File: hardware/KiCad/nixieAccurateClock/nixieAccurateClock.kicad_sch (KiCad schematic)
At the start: 19 parts, among them J1 Conn_01x02_Pin, J2 Conn_01x02_Pin, J3 Conn_01x02_Pin, J4 Conn_01x02_Pin, SW1 SW_DIP_x08, U1 MCP23008-xSO, U2 pico iCE, U3 LTR-329ALS-01

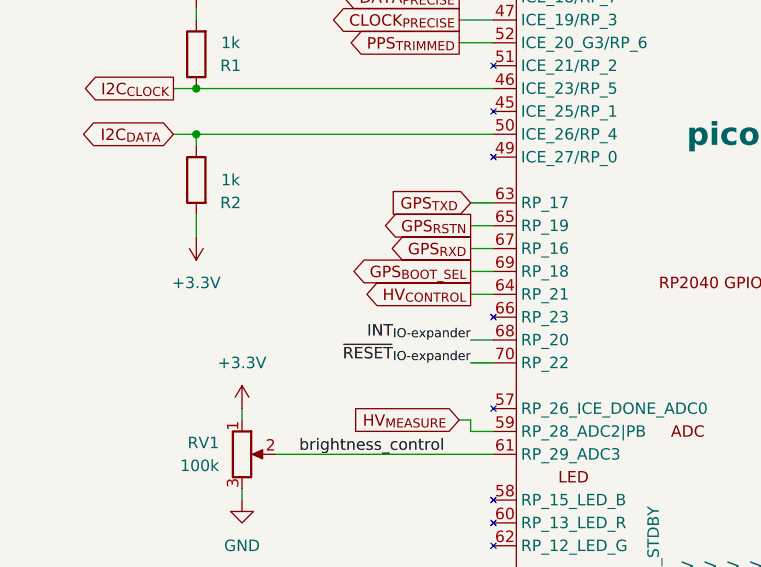
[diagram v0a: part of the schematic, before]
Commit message: WIP pinout config
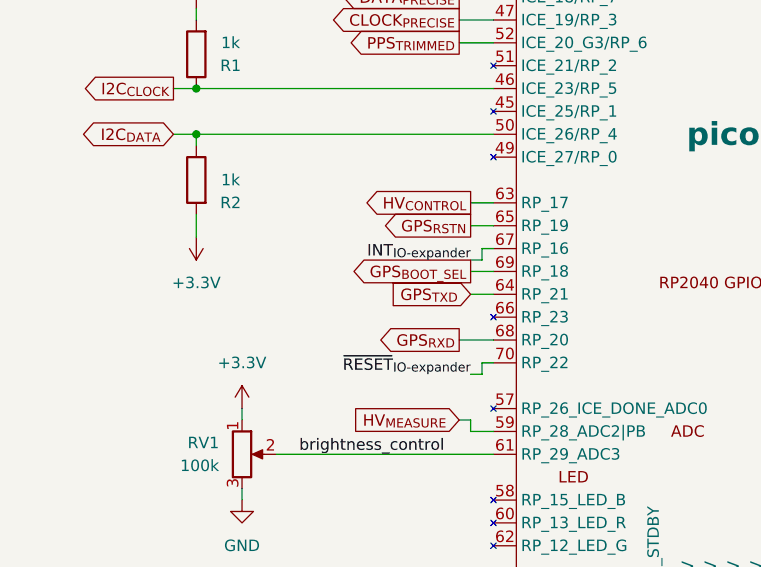
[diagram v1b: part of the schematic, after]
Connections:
- net GPS_{RXD}: now also U2.68 (RP_20); no longer U2.67 (RP_16)
- net GPS_{TXD}: now also U2.64 (RP_21); no longer U2.63 (RP_17)
- net HV_{CONTROL}: now also U2.63 (RP_17); no longer U2.64 (RP_21)
- net INT_{IO-expander}: now also U2.67 (RP_16); no longer U2.68 (RP_20)
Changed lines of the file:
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@@
   (junction (at 114.3 21.59) (diameter 0) (color 0 0 0 0)
   )
+  (wire (pts (xy 73.66 74.93) (xy 73.66 73.66))
+    (stroke (width 0) (type default))
+  )
   (wire (pts (xy 116.84 21.59) (xy 119.38 21.59))
     (stroke (width 0) (type default))
@@
     (stroke (width 0) (type default))
   )
+  (wire (pts (xy 73.66 87.63) (xy 73.66 86.36))
+    (stroke (width 0) (type default))
+  )
   (wire (pts (xy 264.16 34.29) (xy 264.16 36.83))
     (stroke (width 0) (type default))
   )
-  (wire (pts (xy 72.39 83.82) (xy 74.93 83.82))
-    (stroke (width 0) (type default))
-  )
   (wire (pts (xy 207.01 62.23) (xy 207.01 64.77))
     (stroke (width 0) (type default))
@@
     (stroke (width 0) (type default))
   )
+  (wire (pts (xy 72.39 74.93) (xy 73.66 74.93))
+    (stroke (width 0) (type default))
+  )
   (wire (pts (xy 149.86 96.52) (xy 137.16 96.52))
     (stroke (width 0) (type default))
@@
     (stroke (width 0) (type default))
   )
+  (wire (pts (xy 73.66 73.66) (xy 74.93 73.66))
+    (stroke (width 0) (type default))
+  )
   (wire (pts (xy 191.77 49.53) (xy 194.31 49.53))
     (stroke (width 0) (type default))
@@
     (stroke (width 0) (type default))
   )
+  (wire (pts (xy 72.39 78.74) (xy 74.93 78.74))
+    (stroke (width 0) (type default))
+  )
   (wire (pts (xy 92.71 137.16) (xy 92.71 140.97))
     (stroke (width 0) (type default))
@@
     (stroke (width 0) (type default))
   )
-  (wire (pts (xy 72.39 73.66) (xy 74.93 73.66))
-    (stroke (width 0) (type default))
-  )
   (wire (pts (xy 114.3 21.59) (xy 116.84 21.59))
     (stroke (width 0) (type default))
@@
     (stroke (width 0) (type default))
   )
-  (wire (pts (xy 72.39 86.36) (xy 74.93 86.36))
+  (wire (pts (xy 72.39 87.63) (xy 73.66 87.63))
     (stroke (width 0) (type default))
   )
@@
     (stroke (width 0) (type default))
   )
+  (wire (pts (xy 73.66 86.36) (xy 74.93 86.36))
+    (stroke (width 0) (type default))
+  )
+  (wire (pts (xy 71.12 83.82) (xy 74.93 83.82))
+    (stroke (width 0) (type default))
+  )
   (wire (pts (xy 71.12 45.72) (xy 74.93 45.72))
     (stroke (width 0) (type default))
@@
     (stroke (width 0) (type default))
   )
-  (wire (pts (xy 72.39 78.74) (xy 74.93 78.74))
-    (stroke (width 0) (type default))
-  )
   (wire (pts (xy 99.06 21.59) (xy 99.06 22.86))
     (stroke (width 0) (type default))
@@
     (stroke (width 0) (type default))
   )
+  (wire (pts (xy 46.99 91.44) (xy 46.99 92.71))
+    (stroke (width 0) (type default))
+  )
+  (wire (pts (xy 109.22 21.59) (xy 109.22 22.86))
+    (stroke (width 0) (type default))
+  )
+  (wire (pts (xy 106.68 118.11) (xy 109.22 118.11))
+    (stroke (width 0) (type default))
+  )
+  (wire (pts (xy 101.6 21.59) (xy 101.6 22.86))
+    (stroke (width 0) (type default))
+  )
+  (wire (pts (xy 104.14 118.11) (xy 106.68 118.11))
+    (stroke (width 0) (type default))
+  )
+  (wire (pts (xy 261.62 41.91) (xy 264.16 41.91))
+    (stroke (width 0) (type default))
+  )
+  (wire (pts (xy 114.3 21.59) (xy 114.3 22.86))
+    (stroke (width 0) (type default))
+  )
+  (wire (pts (xy 50.8 96.52) (xy 74.93 96.52))
+    (stroke (width 0) (type default))
+  )
+  (wire (pts (xy 190.5 123.19) (xy 190.5 119.38))
+    (stroke (width 0) (type default))
+  )
+  (wire (pts (xy 261.62 34.29) (xy 264.16 34.29))
+    (stroke (width 0) (type default))
+  )
+  (wire (pts (xy 104.14 116.84) (xy 104.14 118.11))
+    (stroke (width 0) (type default))
+  )
   (wire (pts (xy 72.39 68.58) (xy 74.93 68.58))
-    (stroke (width 0) (type default))
-  )
-  (wire (pts (xy 46.99 91.44) (xy 46.99 92.71))
-    (stroke (width 0) (type default))
-  )
-  (wire (pts (xy 109.22 21.59) (xy 109.22 22.86))
-    (stroke (width 0) (type default))
-  )
-  (wire (pts (xy 106.68 118.11) (xy 109.22 118.11))
-    (stroke (width 0) (type default))
-  )
-  (wire (pts (xy 101.6 21.59) (xy 101.6 22.86))
-    (stroke (width 0) (type default))
-  )
-  (wire (pts (xy 104.14 118.11) (xy 106.68 118.11))
-    (stroke (width 0) (type default))
-  )
-  (wire (pts (xy 261.62 41.91) (xy 264.16 41.91))
-    (stroke (width 0) (type default))
-  )
-  (wire (pts (xy 114.3 21.59) (xy 114.3 22.86))
-    (stroke (width 0) (type default))
-  )
-  (wire (pts (xy 50.8 96.52) (xy 74.93 96.52))
-    (stroke (width 0) (type default))
-  )
-  (wire (pts (xy 190.5 123.19) (xy 190.5 119.38))
-    (stroke (width 0) (type default))
-  )
-  (wire (pts (xy 261.62 34.29) (xy 264.16 34.29))
-    (stroke (width 0) (type default))
-  )
-  (wire (pts (xy 104.14 116.84) (xy 104.14 118.11))
     (stroke (width 0) (type default))
   )
@@
     (effects (font (size 1.27 1.27)) (justify right bottom))
   )
-  (label "INT_{IO-expander}" (at 72.39 83.82 180) (fields_autoplaced)
+  (label "INT_{IO-expander}" (at 72.39 74.93 180) (fields_autoplaced)
     (effects (font (size 1.27 1.27)) (justify right bottom))
   )
@@
     (effects (font (size 1.27 1.27)) (justify right bottom))
   )
-  (label "~{RESET}_{IO-expander}" (at 72.39 86.36 180) (fields_autoplaced)
+  (label "~{RESET}_{IO-expander}" (at 72.39 87.63 180) (fields_autoplaced)
     (effects (font (size 1.27 1.27)) (justify right bottom))
   )
@@
     )
   )
-  (global_label "HV_{CONTROL}" (shape output) (at 72.39 78.74 180) (fields_autoplaced)
-    (effects (font (size 1.27 1.27)) (justify right))
-    (property "Intersheetrefs" "${INTERSHEET_REFS}" (at 60.1131 78.74 0)
+  (global_label "HV_{CONTROL}" (shape output) (at 72.39 68.58 180) (fields_autoplaced)
+    (effects (font (size 1.27 1.27)) (justify right))
+    (property "Intersheetrefs" "${INTERSHEET_REFS}" (at 60.1131 68.58 0)
       (effects (font (size 1.27 1.27)) (justify right) hide)
     )
@@
     )
   )
-  (global_label "GPS_{TXD}" (shape input) (at 72.39 68.58 180) (fields_autoplaced)
-    (effects (font (size 1.27 1.27)) (justify right))
-    (property "Intersheetrefs" "${INTERSHEET_REFS}" (at 62.8468 68.58 0)
+  (global_label "GPS_{TXD}" (shape input) (at 72.39 78.74 180) (fields_autoplaced)
+    (effects (font (size 1.27 1.27)) (justify right))
+    (property "Intersheetrefs" "${INTERSHEET_REFS}" (at 62.8468 78.74 0)
       (effects (font (size 1.27 1.27)) (justify right) hide)
     )
@@
     )
   )
-  (global_label "GPS_{RXD}" (shape output) (at 72.39 73.66 180) (fields_autoplaced)
-    (effects (font (size 1.27 1.27)) (justify right))
-    (property "Intersheetrefs" "${INTERSHEET_REFS}" (at 62.6049 73.66 0)
-      (effects (font (size 1.27 1.27)) (justify right) hide)
-    )
+  (global_label "GPS_{RXD}" (shape output) (at 71.12 83.82 180) (fields_autoplaced)
+    (effects (font (size 1.27 1.27)) (justify right))
+    (property "Intersheetrefs" "${INTERSHEET_REFS}" (at 61.3349 83.82 0)
+      (effects (font (size 1.27 1.27)) (justify right) hide)
+    )

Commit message: switch all components to SMT
layout is a mess
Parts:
- J1, J2, J3, J4, J?: footprint Connector_PinHeader_2.54mm:PinHeader_1x02_P2.54mm_Vertical -> Connector_PinHeader_2.54mm:PinHeader_1x02_P2.54mm_Vertical_SMD_Pin1Left; Digikey link https://www.digikey.com/en/products/detail/adam-tech/PH1-02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 -> https://www.digikey.com/en/products/detail/samtec-inc/TSM-1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; Model PH1-02-UA -> TSM-102-01-L-SV; Mouser link https://www.mouser.com/ProductDetail/Samtec/TSW-102-07-G-S?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 -> https://www.mouser.com/ProductDetail/Samtec/TSM-102-01-L-SV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; Price 0.10 -> 0.42
- RV1: footprint Potentiometer_THT:Potentiometer_Bourns_3266Z_Horizontal -> Potentiometer_SMD:Potentiometer_Bourns_3269X_Horizontal; Digikey link https://www.digikey.com/en/products/detail/bourns-inc/3266Z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 -> https://www.digikey.com/en/products/detail/bourns-inc/3269X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; Model 3266Z-1-104LF -> 3269X-1-104GLF; Mouser link https://www.mouser.com/ProductDetail/Bourns/3266Z-1-104LF?q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 -> https://www.mouser.com/ProductDetail/Bourns/3269X-1-104GLF?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; Price 4.20 -> 3.68

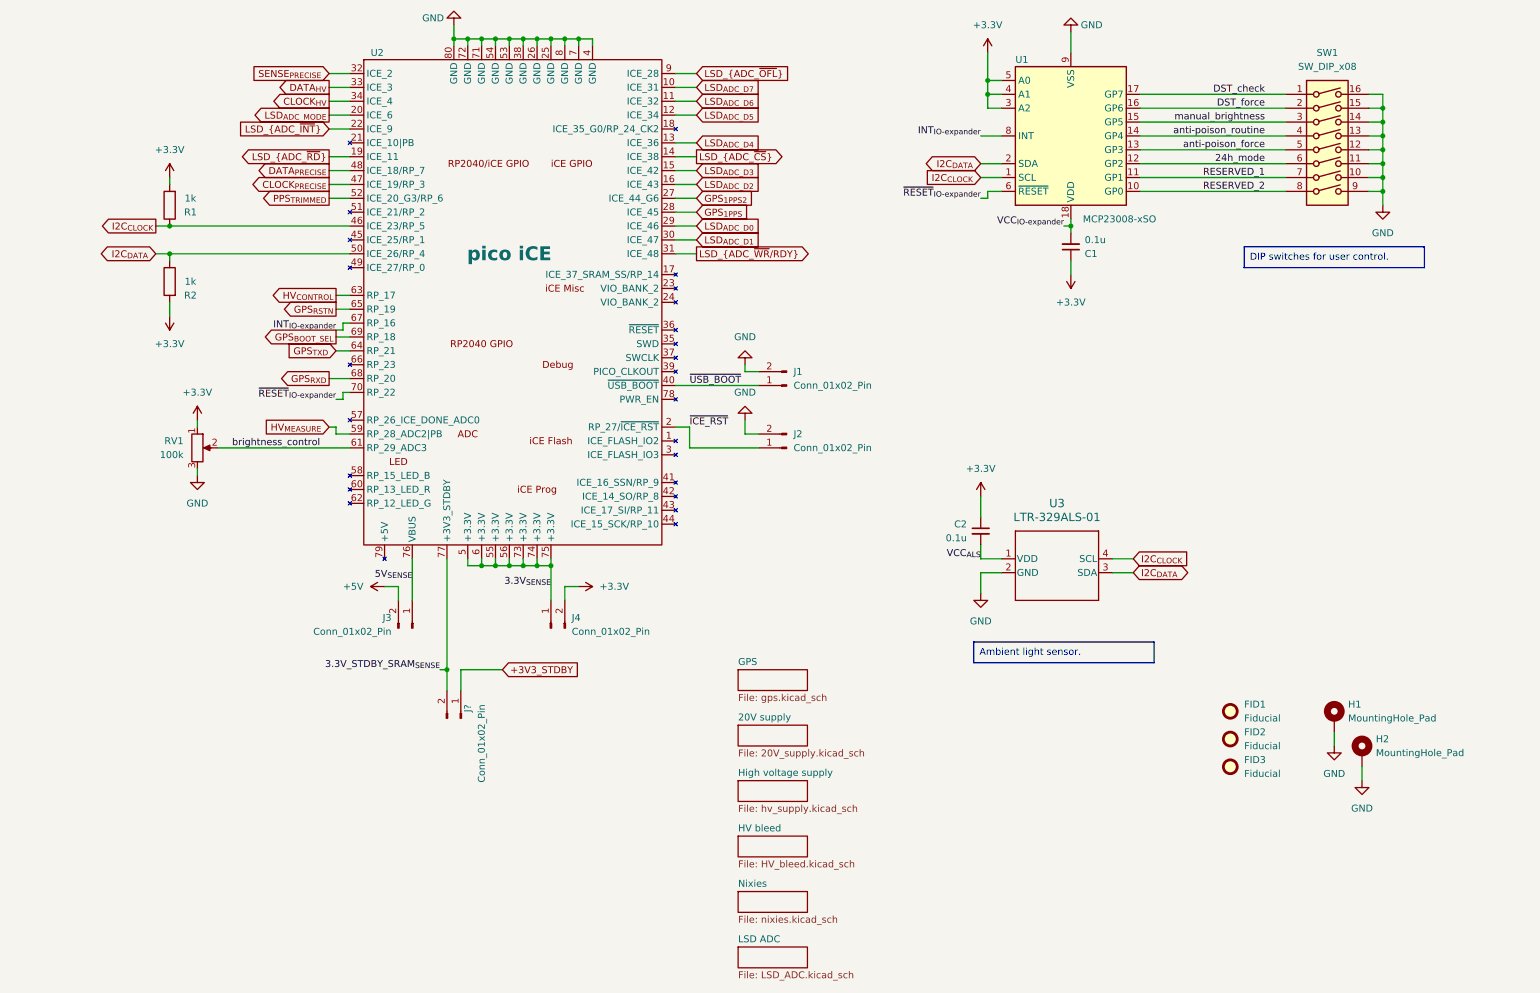
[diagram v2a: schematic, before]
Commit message: switch to all SM components
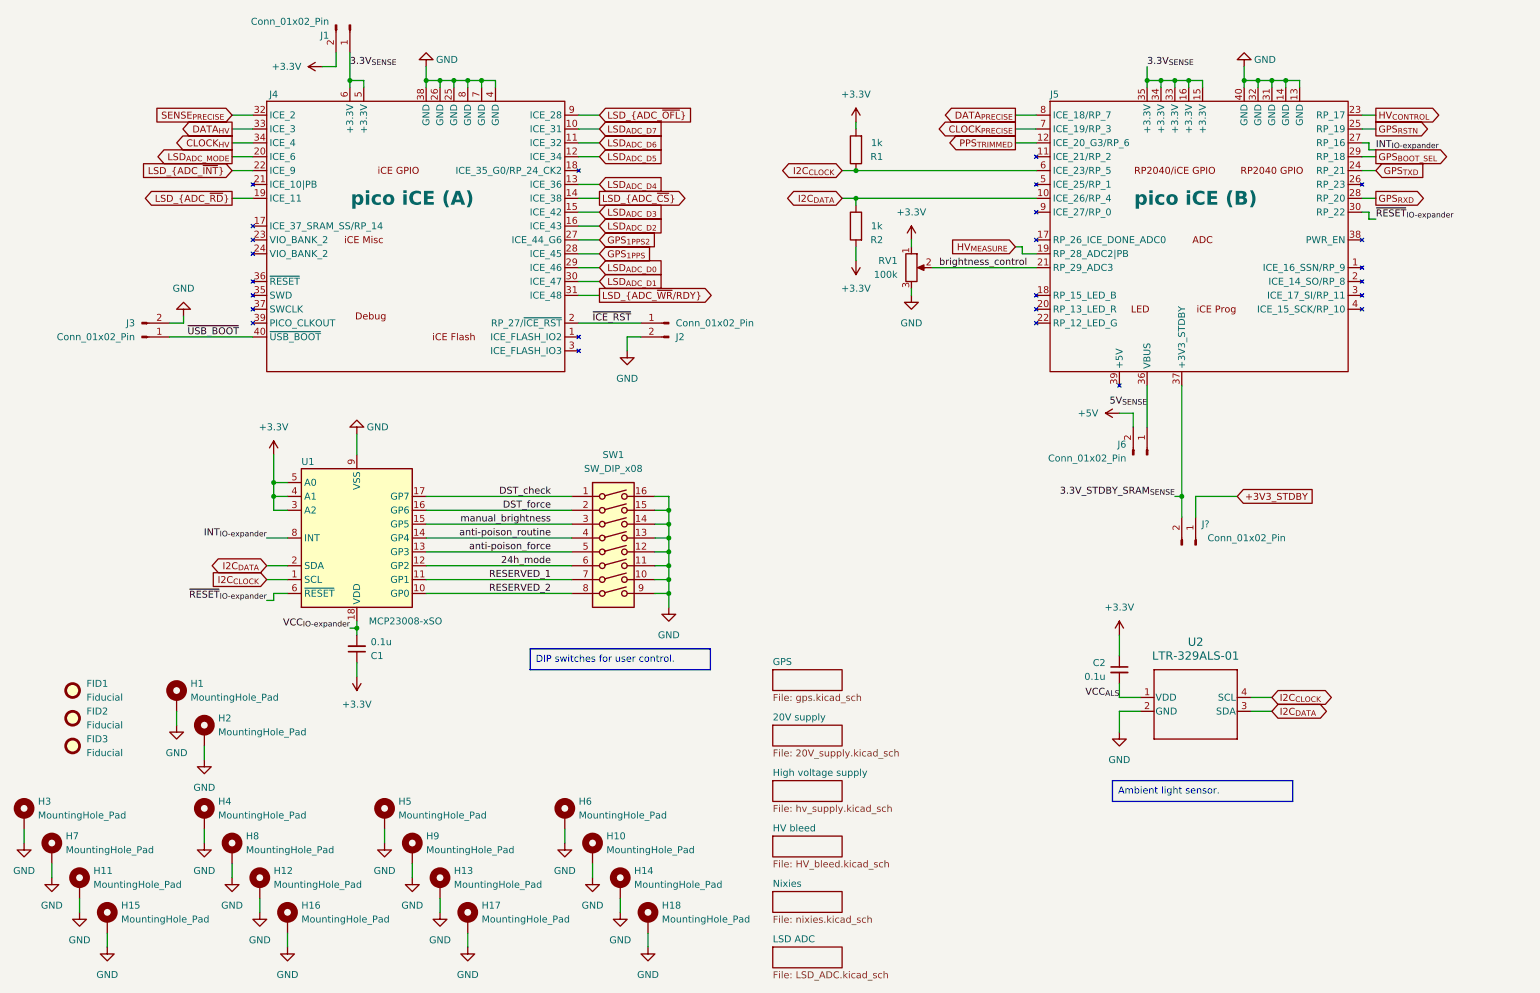
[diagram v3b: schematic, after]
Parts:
- removed J4, J?: Conn_01x02_Pin, Connector_PinHeader_2.54mm:PinHeader_1x02_P2.54mm_Vertical_SMD_Pin1Left, symbol Connector:Conn_01x02_Pin
- removed U2: pico iCE, 00_lib:pico iCE, symbol 00_lib:pico_iCE
- added H10, H11, H12, H13, H14, H15, H16, H17, H18, H3, H4, H5, H6, H7, H8, H9: MountingHole_Pad, MountingHole:MountingHole_2.7mm_M2.5_Pad_Via, symbol Mechanical:MountingHole_Pad
- added J4: pico iCE (A), 00_lib:pico iCE (A), symbol 00_lib:pico_iCE (A)
- added J5: pico iCE (B), 00_lib:pico iCE (B), symbol 00_lib:pico_iCE (B)
- added J6, J?: Conn_01x02_Pin, Connector_PinHeader_2.54mm:PinHeader_1x02_P2.54mm_Vertical_SMD_Pin1Left, symbol Connector:Conn_01x02_Pin
- renumbered U3 to U2
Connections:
- net +3.3V: now also J1.2 (Pin_2)
- net +3V3_STDBY: now also J?.1 (Pin_1)
- net +5V: now also J6.2 (Pin_2); no longer J3.2 (Pin_2)
- net 3.3V_STDBY_SRAM_{SENSE}: now also J5.37 (+3V3_STDBY), J?.2 (Pin_2)
- net 3.3V_{SENSE}: now also J1.1 (Pin_1), J4.5 (+3.3V), J4.6 (+3.3V), J5.15 (+3.3V), J5.16 (+3.3V), J5.33 (+3.3V), J5.34 (+3.3V), J5.35 (+3.3V)
- net 5V_{SENSE}: now also J5.36 (VBUS), J6.1 (Pin_1); no longer J3.1 (Pin_1)
- net CLOCK_{HV}: now also J4.34 (ICE_4)
- net CLOCK_{PRECISE}: now also J5.7 (ICE_19/RP_3)
- net DATA_{HV}: now also J4.33 (ICE_3)
- net DATA_{PRECISE}: now also J5.8 (ICE_18/RP_7)
- net GND: now also J3.2 (Pin_2), H10.1, H11.1, H12.1, H13.1, H14.1, H15.1, H16.1, H17.1, H18.1, H3.1, H4.1, H5.1, H6.1, H7.1, H8.1, H9.1, J4.25 (GND), J4.26 (GND), J4.38 (GND), J4.4 (GND), J4.7 (GND), J4.8 (GND), J5.13 (GND), J5.14 (GND), J5.31 (GND), J5.32 (GND), J5.40 (GND); no longer J1.2 (Pin_2)
- net GPS_{1PPS2}: now also J4.27 (ICE_44_G6)
- net GPS_{1PPS}: now also J4.28 (ICE_45)
- net GPS_{BOOT_SEL}: now also J5.29 (RP_18)
- net GPS_{RSTN}: now also J5.25 (RP_19)
- net GPS_{RXD}: now also J5.28 (RP_20)
- net GPS_{TXD}: now also J5.24 (RP_21)
- net HV_{CONTROL}: now also J5.23 (RP_17)
- net HV_{MEASURE}: now also J5.19 (RP_28_ADC2|PB)
- net I2C_{CLOCK}: now also J5.6 (ICE_23/RP_5)
- net I2C_{DATA}: now also J5.10 (ICE_26/RP_4)
- net INT_{IO-expander}: now also J5.27 (RP_16)
- net LSD_{ADC_D0}: now also J4.29 (ICE_46)
- net LSD_{ADC_D1}: now also J4.30 (ICE_47)
- net LSD_{ADC_D2}: now also J4.16 (ICE_43)
- net LSD_{ADC_D3}: now also J4.15 (ICE_42)
- net LSD_{ADC_D4}: now also J4.13 (ICE_36)
- net LSD_{ADC_D5}: now also J4.12 (ICE_34)
- net LSD_{ADC_D6}: now also J4.11 (ICE_32)
- net LSD_{ADC_D7}: now also J4.10 (ICE_31)
- net LSD_{ADC_MODE}: now also J4.20 (ICE_6)
- net LSD_{ADC_~{CS}}: now also J4.14 (ICE_38)
- net LSD_{ADC_~{INT}}: now also J4.22 (ICE_9)
- net LSD_{ADC_~{OFL}}: now also J4.9 (ICE_28)
- net LSD_{ADC_~{RD}}: now also J4.19 (ICE_11)
- net LSD_{ADC_~{WR}/RDY}: now also J4.31 (ICE_48)
- net PPS_{TRIMMED}: now also J5.12 (ICE_20_G3/RP_6)
- net SENSE_{PRECISE}: now also J4.32 (ICE_2)
- net brightness_control: now also J5.21 (RP_29_ADC3)
- net ~{ICE_RST}: now also J4.2 (RP_27/~{ICE_RST})
- net ~{RESET}_{IO-expander}: now also J5.30 (RP_22)
- net ~{USB_BOOT}: now also J3.1 (Pin_1), J4.40 (~{USB_BOOT}); no longer J1.1 (Pin_1)
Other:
- moved on the sheet: C1, C2, FID1, FID2, FID3, H1, H2, SW1, U1, U2

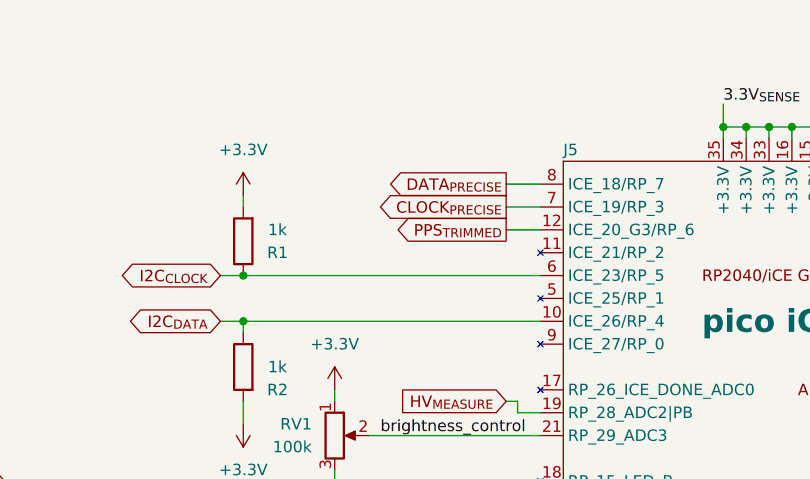
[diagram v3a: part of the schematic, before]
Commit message: switch to static level shifting
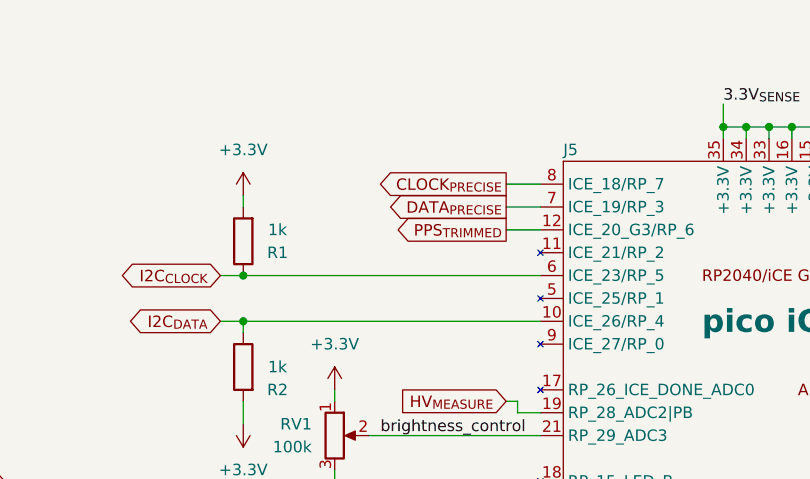
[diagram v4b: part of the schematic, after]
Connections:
- net CLOCK_{PRECISE}: now also J5.8 (ICE_18/RP_7); no longer J5.7 (ICE_19/RP_3)
- net DATA_{PRECISE}: now also J5.7 (ICE_19/RP_3); no longer J5.8 (ICE_18/RP_7)
